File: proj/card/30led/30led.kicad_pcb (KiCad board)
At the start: 2 copper layers, 100 x 75 mm, 53 parts, among them J1 UPDI, J2 USB_C_Receptacle_USB2.0_16P, SW1 SW_Push, SW2 SW_Push, U1 ATtiny404-SS, U2 CH340K

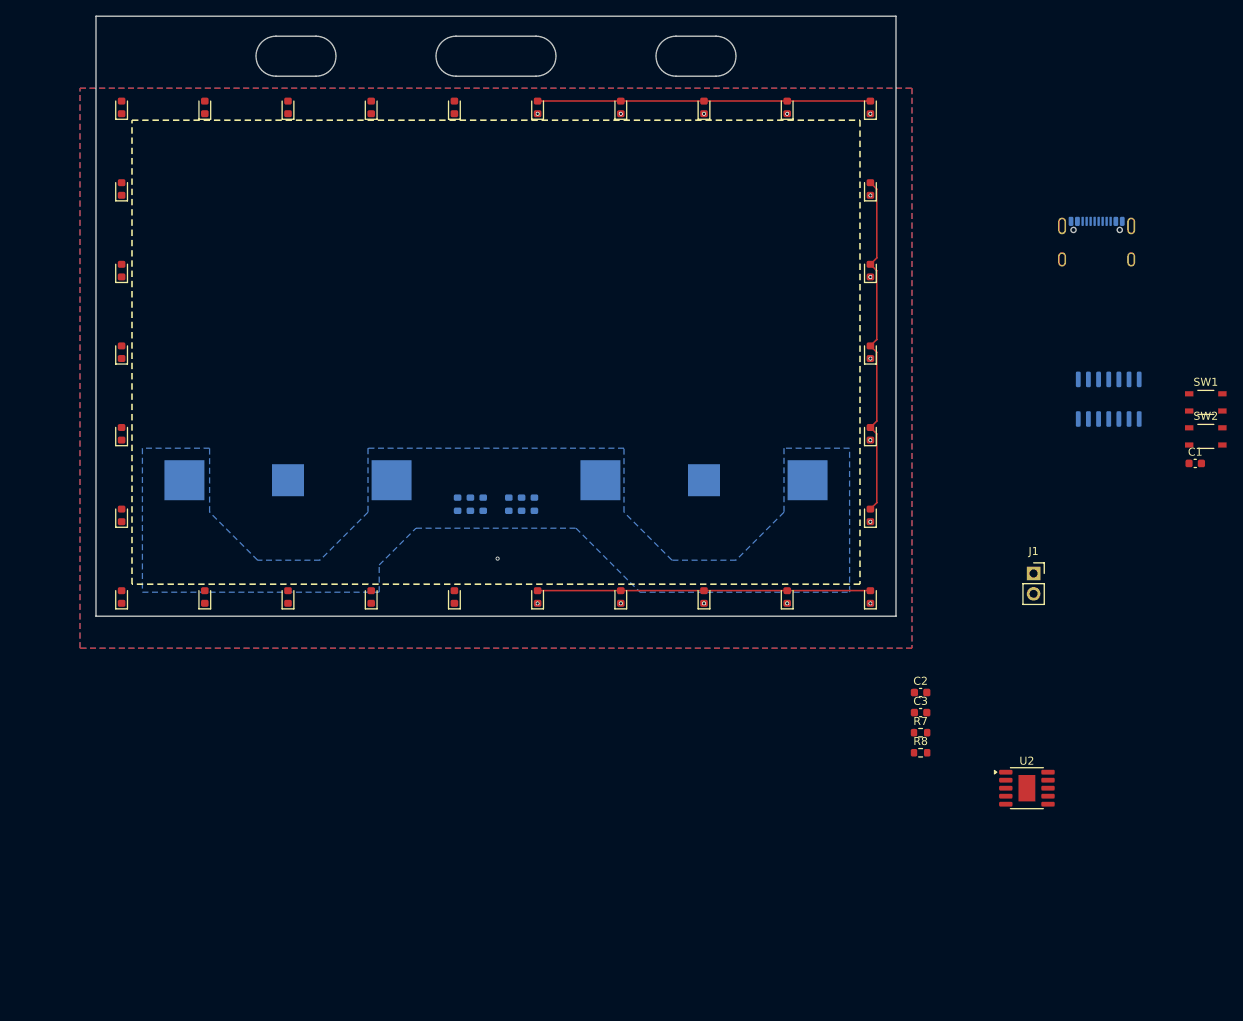
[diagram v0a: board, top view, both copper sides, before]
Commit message: -
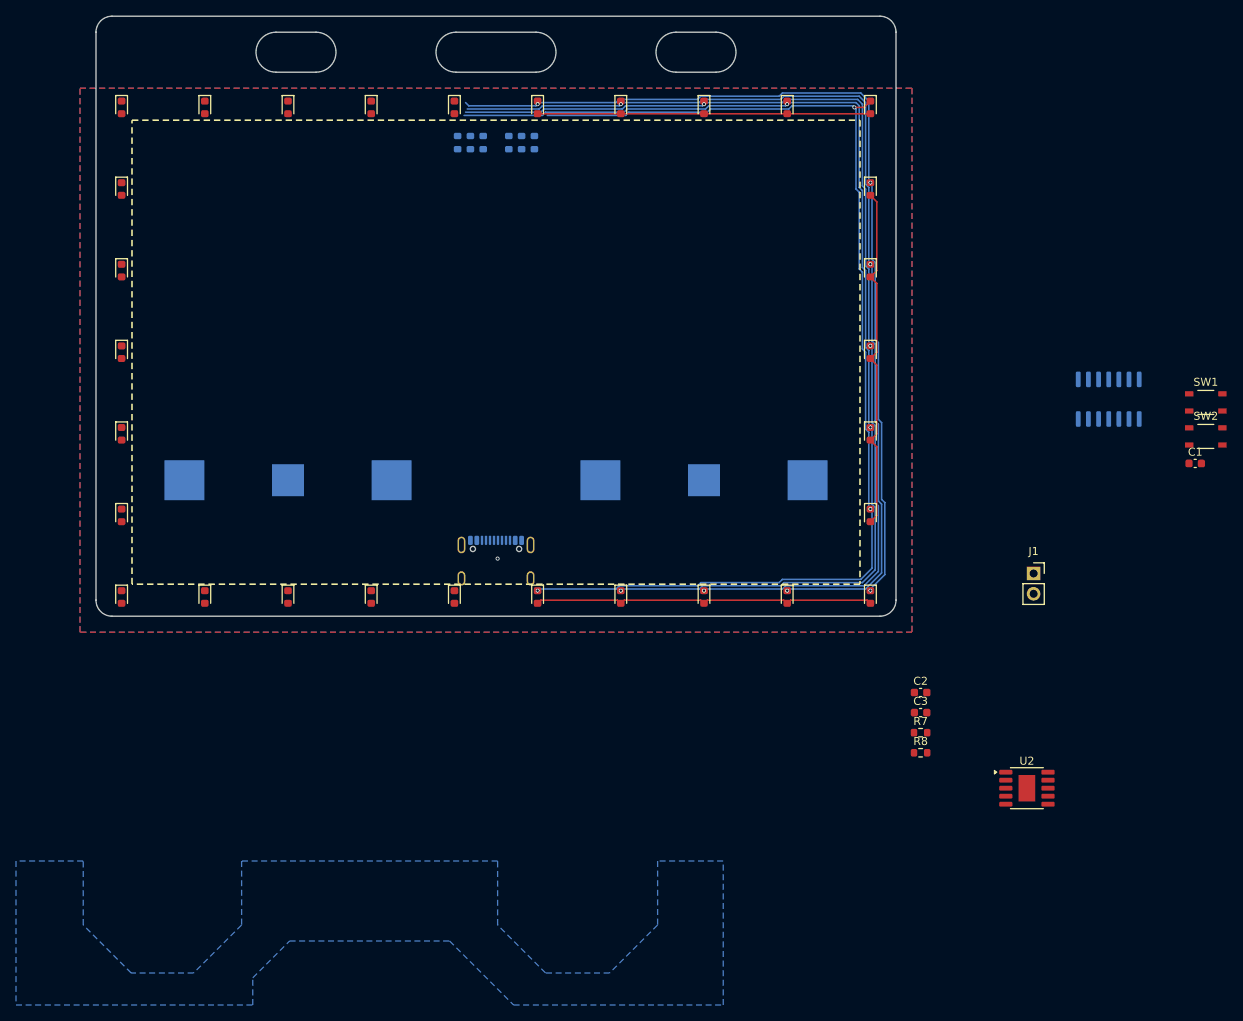
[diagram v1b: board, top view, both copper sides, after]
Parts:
- moved J2 85.0 mm to (100.0, 127.2)
- moved R3 46.2 mm to (95.2, 73.8), turned to 90 degrees
- moved R4 46.2 mm to (104.8, 73.8), turned to 90 degrees
- moved R2 45.7 mm to (96.8, 73.8), turned to 90 degrees
- moved R5 45.7 mm to (103.2, 73.8), turned to 90 degrees
- moved R1 45.3 mm to (98.4, 73.8), turned to 90 degrees
- moved R6 45.3 mm to (101.6, 73.8), turned to 90 degrees
- turned D1 to -90 degrees
- turned D10 to -90 degrees
- turned D11 to -90 degrees
- turned D12 to -90 degrees
- turned D13 to -90 degrees
- turned D14 to -90 degrees
- turned D15 to -90 degrees
- turned D16 to -90 degrees
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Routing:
- net ROW5: track 0.00 -> 142.8 mm
- net ROW4: track 0.00 -> 141.9 mm
- net ROW3: track 0.00 -> 132.5 mm
- net ROW2: track 0.00 -> 123.1 mm
- net ROW1: track 0.00 -> 114.4 mm
- net /_COL1: track 41.6 -> 43.0 mm
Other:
- outline, holes or cut-outs redrawn
- board text added: "${REFERENCE}"
